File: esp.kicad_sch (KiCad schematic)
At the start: 26 parts, among them J1 Barrel_Jack, J3 Barrel_Jack, J4 Barrel_Jack, J5 Barrel_Jack, J7 Barrel_Jack_MountingPin, P1 Conn_WallPlug_Earth, U1 ESP32-S2-WROVER, U14 PCF8574ATS, U16 L298N, U17 PCA9685PW, U18 NID30S48-24, U2 TCA9548ARGER, U3 TCA9548ARGER, U4 BME280, U5 CCS811, U6 PCF8574ATS, U7 OKI-78SR-12_1.0-W36H-C, U8 OKI-78SR-5_1.5-W36-C, U9 OKI-78SR-3.3_1.5-W36H-C

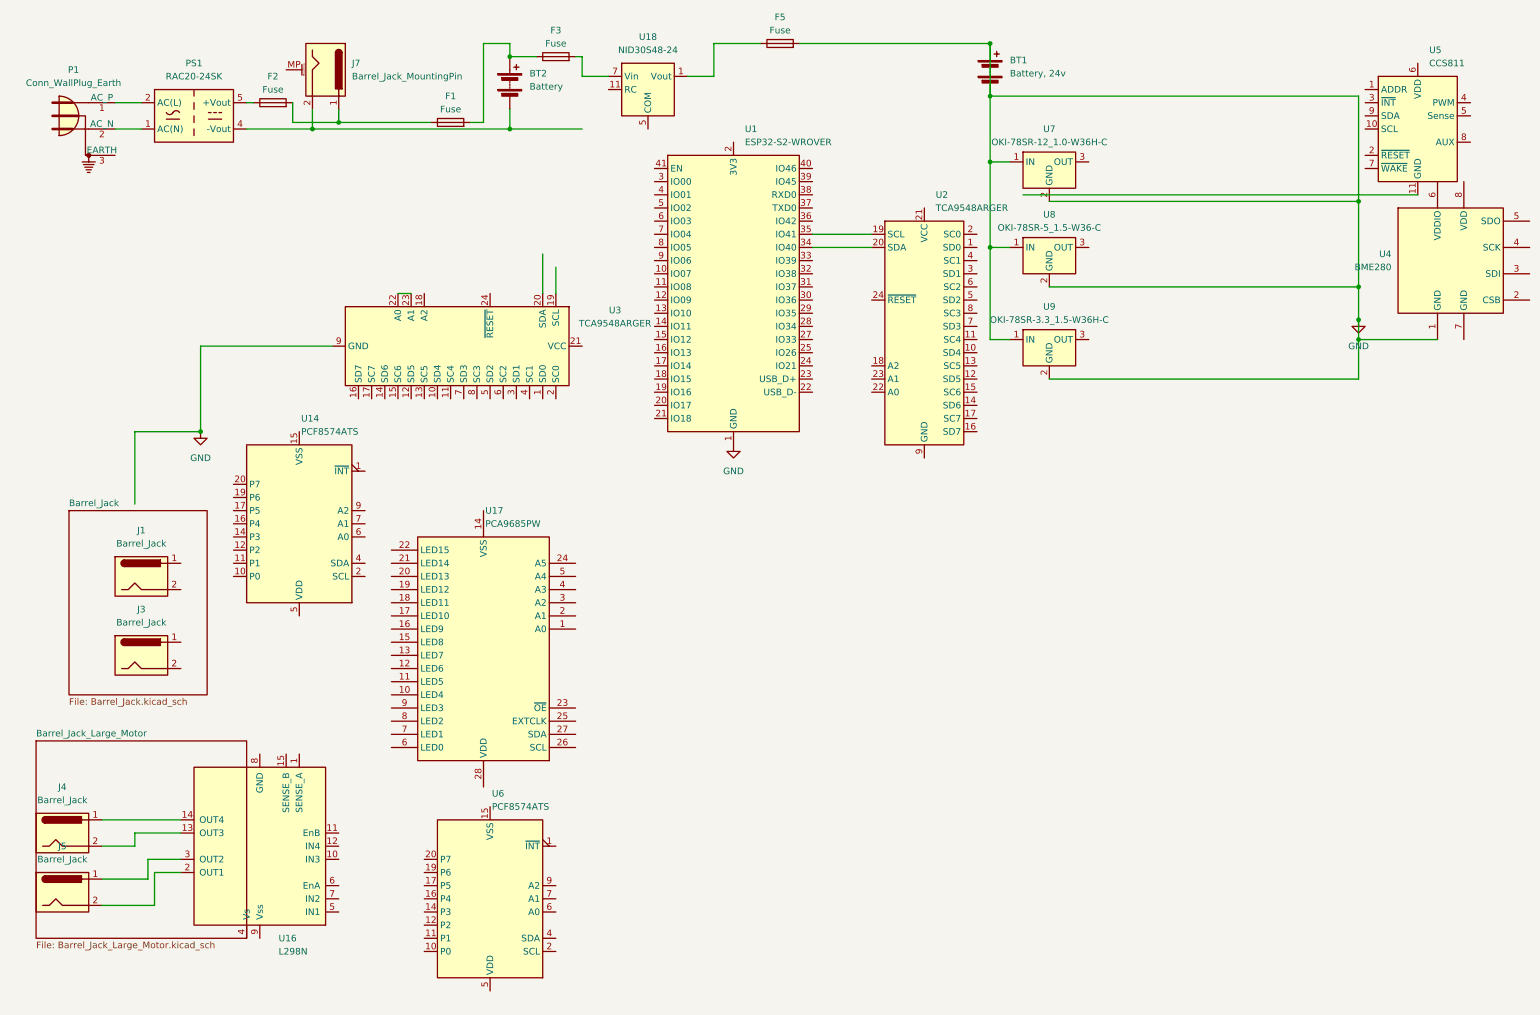
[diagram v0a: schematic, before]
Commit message: motor layout
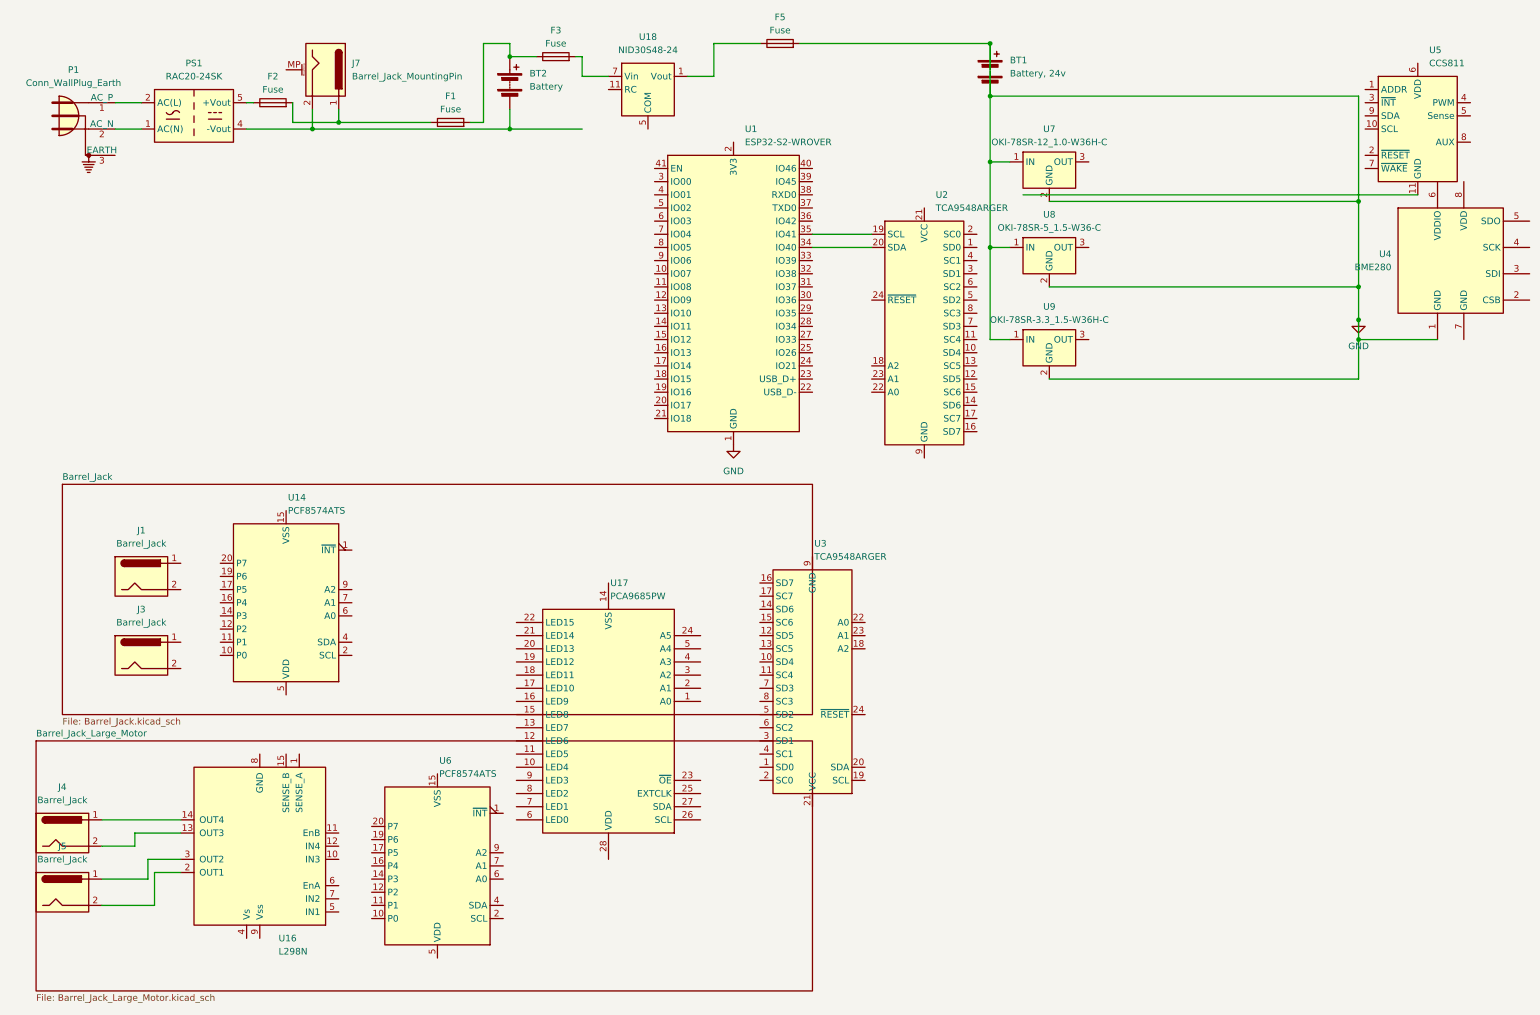
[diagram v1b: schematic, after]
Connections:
- net GND: no longer U3.9 (GND)
- net at U3.22 (A0): no longer U3.23 (A1)
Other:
- moved on the sheet: U14, U17, U3, U6
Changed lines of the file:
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@@
   (junction (at 66.04 30.48) (diameter 0) (color 0 0 0 0)
   )
-  (junction (at 44.45 88.9) (diameter 0) (color 0 0 0 0)
-  )
   (junction (at 267.97 60.96) (diameter 0) (color 0 0 0 0)
   )
@@
     (stroke (width 0) (type default))
   )
-  (wire (pts (xy 82.55 62.23) (xy 85.09 62.23))
-    (stroke (width 0) (type default))
-  )
   (wire (pts (xy 196.85 24.13) (xy 196.85 36.83))
     (stroke (width 0) (type default))
@@
     (stroke (width 0) (type default))
   )
-  (wire (pts (xy 31.75 88.9) (xy 31.75 102.87))
-    (stroke (width 0) (type default))
-  )
-  (wire (pts (xy 31.75 88.9) (xy 44.45 88.9))
-    (stroke (width 0) (type default))
-  )
   (wire (pts (xy 31.75 168.91) (xy 25.4 168.91))
     (stroke (width 0) (type default))
@@
     (stroke (width 0) (type default))
   )
-  (wire (pts (xy 69.85 72.39) (xy 44.45 72.39))
-    (stroke (width 0) (type default))
-  )
   (wire (pts (xy 162.56 50.8) (xy 173.99 50.8))
     (stroke (width 0) (type default))
@@
     (stroke (width 0) (type default))
   )
-  (wire (pts (xy 44.45 72.39) (xy 44.45 88.9))
-    (stroke (width 0) (type default))
-  )
   (wire (pts (xy 267.97 71.12) (xy 267.97 78.74))
     (stroke (width 0) (type default))
@@
     (stroke (width 0) (type default))
   )
-  (wire (pts (xy 110.49 62.23) (xy 110.49 54.61))
-    (stroke (width 0) (type default))
-  )
   (wire (pts (xy 27.94 25.4) (xy 33.02 25.4))
     (stroke (width 0) (type default))
@@
   )
   (wire (pts (xy 53.34 25.4) (xy 54.61 25.4))
-    (stroke (width 0) (type default))
-  )
-  (wire (pts (xy 113.03 62.23) (xy 113.03 57.15))
     (stroke (width 0) (type default))
   )
@@
     )
   )
-  (symbol (lib_id "Driver_LED:PCA9685PW") (at 99.06 132.08 180) (unit 1)
-    (in_bom yes) (on_board yes) (dnp no) (fields_autoplaced)
-    (property "Reference" "U17" (at 99.4059 104.14 0)
-      (effects (font (size 1.27 1.27)) (justify right))
-    )
-    (property "Value" "PCA9685PW" (at 99.4059 106.68 0)
-      (effects (font (size 1.27 1.27)) (justify right))
-    )
-    (property "Footprint" "Package_SO:TSSOP-28_4.4x9.7mm_P0.65mm" (at 98.425 107.315 0)
+  (symbol (lib_id "Driver_LED:PCA9685PW") (at 123.19 146.05 180) (unit 1)
+    (in_bom yes) (on_board yes) (dnp no) (fields_autoplaced)
+    (property "Reference" "U17" (at 123.5359 118.11 0)
+      (effects (font (size 1.27 1.27)) (justify right))
+    )
+    (property "Value" "PCA9685PW" (at 123.5359 120.65 0)
+      (effects (font (size 1.27 1.27)) (justify right))
+    )
+    (property "Footprint" "Package_SO:TSSOP-28_4.4x9.7mm_P0.65mm" (at 122.555 121.285 0)
       (effects (font (size 1.27 1.27)) (justify left) hide)
     )
-    (property "Datasheet" "http://www.nxp.com/docs/en/data-sheet/PCA9685.pdf" (at 109.22 149.86 0)
+    (property "Datasheet" "http://www.nxp.com/docs/en/data-sheet/PCA9685.pdf" (at 133.35 163.83 0)
       (effects (font (size 1.27 1.27)) hide)
     )
@@
     )
   )
-  (symbol (lib_id "Interface_Expansion:TCA9548ARGER") (at 95.25 72.39 270) (unit 1)
-    (in_bom yes) (on_board yes) (dnp no) (fields_autoplaced)
-    (property "Reference" "U3" (at 124.46 65.4619 90)
-      (effects (font (size 1.27 1.27)))
-    )
-    (property "Value" "TCA9548ARGER" (at 124.46 68.0019 90)
-      (effects (font (size 1.27 1.27)))
-    )
-    (property "Footprint" "Package_DFN_QFN:Texas_RGE0024C_EP2.1x2.1mm" (at 69.85 72.39 0)
-      (effects (font (size 1.27 1.27)) hide)
-    )
-    (property "Datasheet" "http://www.ti.com/lit/ds/symlink/tca9548a.pdf" (at 101.6 73.66 0)
+  (symbol (lib_id "Interface_Expansion:TCA9548ARGER") (at 162.56 138.43 180) (unit 1)
+    (in_bom yes) (on_board yes) (dnp no) (fields_autoplaced)
+    (property "Reference" "U3" (at 162.9059 110.49 0)
+      (effects (font (size 1.27 1.27)) (justify right))
+    )
+    (property "Value" "TCA9548ARGER" (at 162.9059 113.03 0)
+      (effects (font (size 1.27 1.27)) (justify right))
+    )
+    (property "Footprint" "Package_DFN_QFN:Texas_RGE0024C_EP2.1x2.1mm" (at 162.56 113.03 0)
+      (effects (font (size 1.27 1.27)) hide)
+    )
+    (property "Datasheet" "http://www.ti.com/lit/ds/symlink/tca9548a.pdf" (at 161.29 144.78 0)
       (effects (font (size 1.27 1.27)) hide)
     )
@@
     )
   )
-  (symbol (lib_id "power:GND") (at 44.45 88.9 0) (unit 1)
-    (in_bom yes) (on_board yes) (dnp no) (fields_autoplaced)
-    (property "Reference" "#PWR02" (at 44.45 95.25 0)
-      (effects (font (size 1.27 1.27)) hide)
-    )
-    (property "Value" "GND" (at 44.45 93.98 0)
-      (effects (font (size 1.27 1.27)))
-    )
-    (property "Footprint" "" (at 44.45 88.9 0)
-      (effects (font (size 1.27 1.27)) hide)
-    )
-    (property "Datasheet" "" (at 44.45 88.9 0)
-      (effects (font (size 1.27 1.27)) hide)
-    )
-    (pin "1")
-    (instances
-      (project "esp"
-        (path "/dab6683c-420f-459a-bf9c-0c28b4b081e3"
-          (reference "#PWR02") (unit 1)
-        )
-      )
-    )
-  )
   (symbol (lib_id "Connector:Conn_WallPlug_Earth") (at 20.32 27.94 0) (unit 1)
     (in_bom yes) (on_board yes) (dnp no) (fields_autoplaced)
@@
     )
   )
-  (symbol (lib_id "Interface_Expansion:PCF8574ATS") (at 100.33 179.07 180) (unit 1)
-    (in_bom yes) (on_board yes) (dnp no) (fields_autoplaced)
-    (property "Reference" "U6" (at 100.6759 158.75 0)
-      (effects (font (size 1.27 1.27)) (justify right))
-    )
-    (property "Value" "PCF8574ATS" (at 100.6759 161.29 0)
-      (effects (font (size 1.27 1.27)) (justify right))
-    )
-    (property "Footprint" "Package_SO:SSOP-20_4.4x6.5mm_P0.65mm" (at 100.33 179.07 0)
-      (effects (font (size 1.27 1.27)) hide)
-    )
-    (property "Datasheet" "http://www.nxp.com/docs/en/data-sheet/PCF8574_PCF8574A.pdf" (at 100.33 179.07 0)
+  (symbol (lib_id "Interface_Expansion:PCF8574ATS") (at 90.17 172.72 180) (unit 1)
+    (in_bom yes) (on_board yes) (dnp no) (fields_autoplaced)
+    (property "Reference" "U6" (at 90.5159 152.4 0)
+      (effects (font (size 1.27 1.27)) (justify right))
+    )
+    (property "Value" "PCF8574ATS" (at 90.5159 154.94 0)
+      (effects (font (size 1.27 1.27)) (justify right))
+    )
+    (property "Footprint" "Package_SO:SSOP-20_4.4x6.5mm_P0.65mm" (at 90.17 172.72 0)
+      (effects (font (size 1.27 1.27)) hide)
+    )
+    (property "Datasheet" "http://www.nxp.com/docs/en/data-sheet/PCF8574_PCF8574A.pdf" (at 90.17 172.72 0)
       (effects (font (size 1.27 1.27)) hide)
     )
@@
     )
   )
-  (symbol (lib_id "Interface_Expansion:PCF8574ATS") (at 63.5 106.68 180) (unit 1)
-    (in_bom yes) (on_board yes) (dnp no) (fields_autoplaced)
-    (property "Reference" "U14" (at 63.8459 86.36 0)
-      (effects (font (size 1.27 1.27)) (justify right))
-    )
-    (property "Value" "PCF8574ATS" (at 63.8459 88.9 0)
-      (effects (font (size 1.27 1.27)) (justify right))
-    )
-    (property "Footprint" "Package_SO:SSOP-20_4.4x6.5mm_P0.65mm" (at 63.5 106.68 0)
-      (effects (font (size 1.27 1.27)) hide)
-    )
-    (property "Datasheet" "http://www.nxp.com/docs/en/data-sheet/PCF8574_PCF8574A.pdf" (at 63.5 106.68 0)
+  (symbol (lib_id "Interface_Expansion:PCF8574ATS") (at 60.96 121.92 180) (unit 1)
+    (in_bom yes) (on_board yes) (dnp no) (fields_autoplaced)
+    (property "Reference" "U14" (at 61.3059 101.6 0)
+      (effects (font (size 1.27 1.27)) (justify right))
+    )
+    (property "Value" "PCF8574ATS" (at 61.3059 104.14 0)
+      (effects (font (size 1.27 1.27)) (justify right))
+    )
+    (property "Footprint" "Package_SO:SSOP-20_4.4x6.5mm_P0.65mm" (at 60.96 121.92 0)
+      (effects (font (size 1.27 1.27)) hide)
+    )
+    (property "Datasheet" "http://www.nxp.com/docs/en/data-sheet/PCF8574_PCF8574A.pdf" (at 60.96 121.92 0)
       (effects (font (size 1.27 1.27)) hide)
     )
@@
     )
   )
-  (sheet (at 12.7 148.59) (size 40.64 38.1) (fields_autoplaced)
+  (sheet (at 12.7 148.59) (size 149.86 48.26) (fields_autoplaced)
     (stroke (width 0.1524) (type solid))
     (fill (color 0 0 0 0.0000))
@@
       (effects (font (size 1.27 1.27)) (justify left bottom))
     )
-    (property "Sheetfile" "Barrel_Jack_Large_Motor.kicad_sch" (at 12.7 187.2746 0)
+    (property "Sheetfile" "Barrel_Jack_Large_Motor.kicad_sch" (at 12.7 197.4346 0)
       (effects (font (size 1.27 1.27)) (justify left top))
     )
@@
     )
   )
-  (sheet (at 19.05 104.14) (size 26.67 35.56) (fields_autoplaced)
+  (sheet (at 17.78 99.06) (size 144.78 44.45) (fields_autoplaced)
     (stroke (width 0.1524) (type solid))
     (fill (color 0 0 0 0.0000))
-    (property "Sheetname" "Barrel_Jack" (at 19.05 103.4284 0)
+    (property "Sheetname" "Barrel_Jack" (at 17.78 98.3484 0)
       (effects (font (size 1.27 1.27)) (justify left bottom))
     )
-    (property "Sheetfile" "Barrel_Jack.kicad_sch" (at 19.05 140.2846 0)
+    (property "Sheetfile" "Barrel_Jack.kicad_sch" (at 17.78 144.0946 0)
       (effects (font (size 1.27 1.27)) (justify left top))
     )
